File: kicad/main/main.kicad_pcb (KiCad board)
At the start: 2 copper layers, 45.7 x 35 mm, 19 parts, among them J2 Conn_01x02, J3 Conn_01x07_Pin, J4 Conn_01x04_Pin, P1 USB_C_Plug_USB2.0, SW1 MK-12C03-G015, SW3 SW_Push, SW4 SW_Push, U1 HUSB237, U2 ZX-PH2.0-WT4P

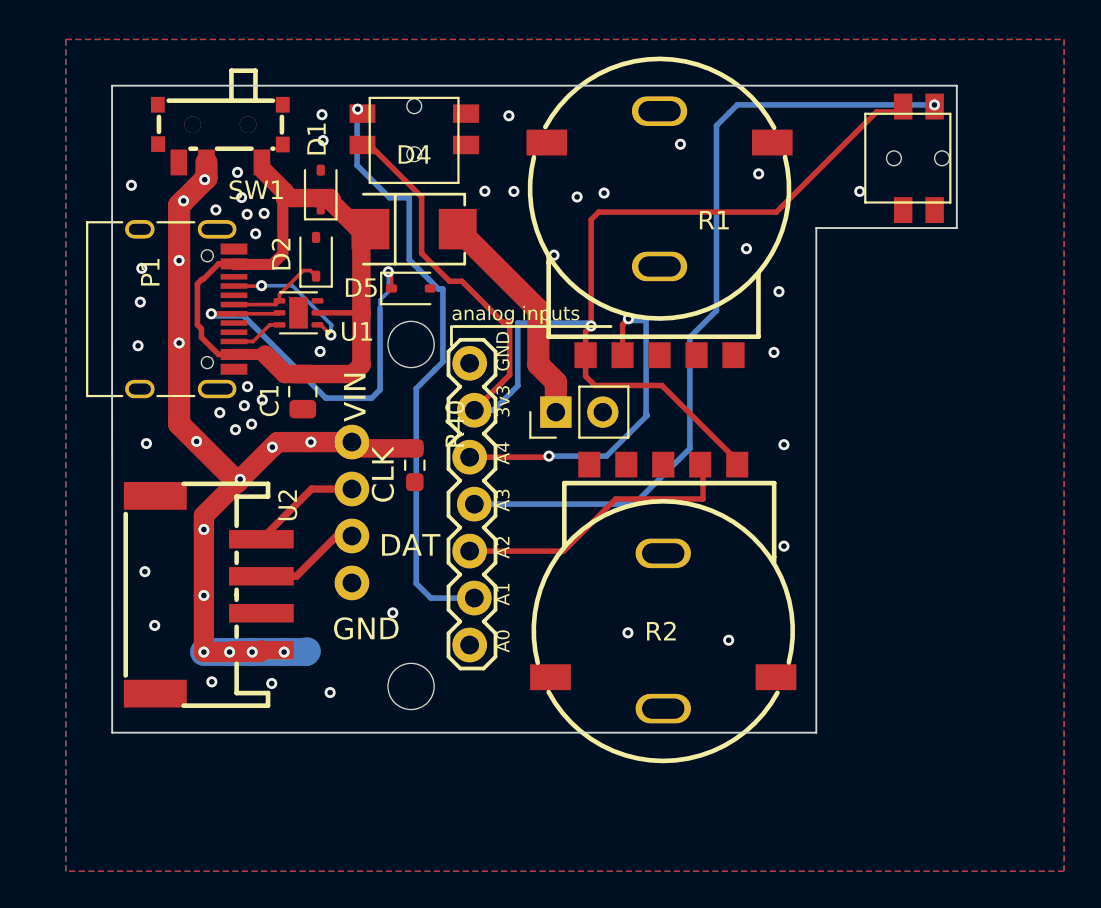
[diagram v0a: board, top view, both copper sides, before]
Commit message: Revamped PCB
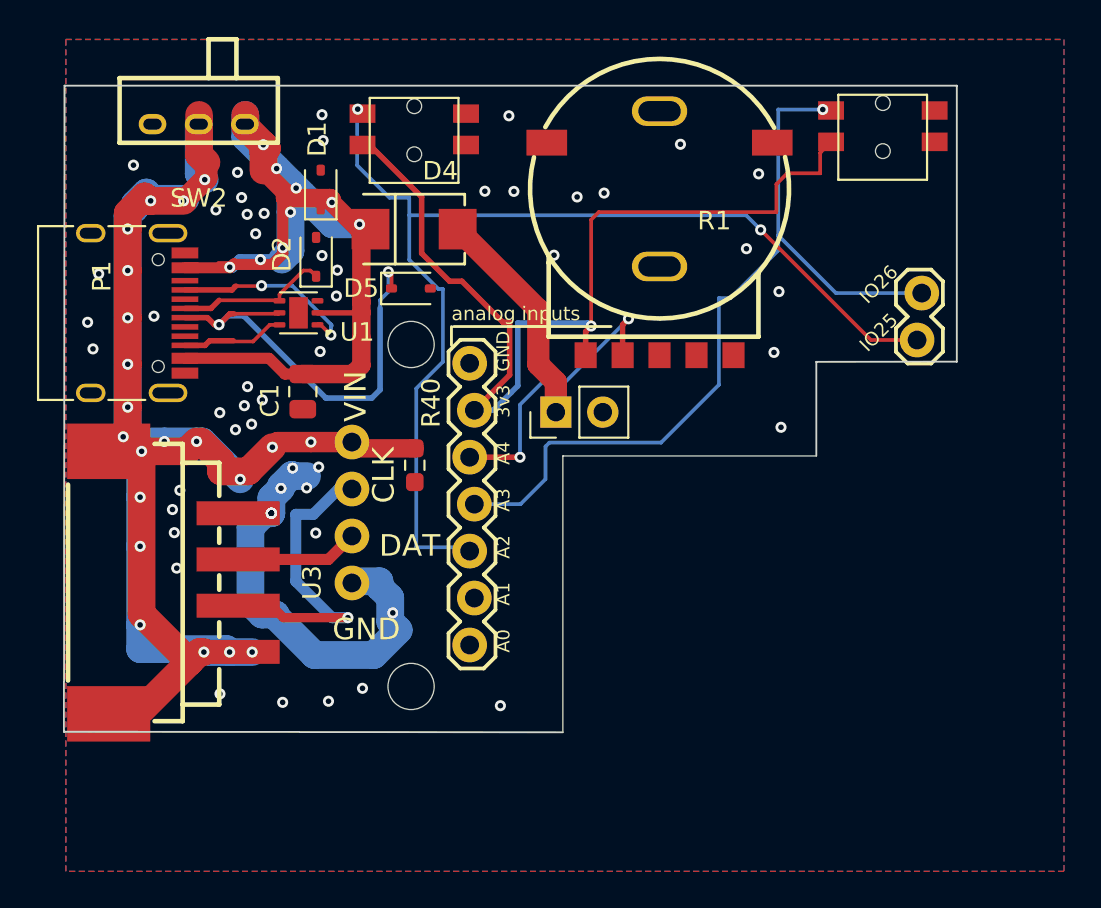
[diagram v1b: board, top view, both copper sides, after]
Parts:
- removed R2: RK10J11R0A0H, easyeda2kicad:RES-SMD_RK10J11R0A0H
- removed SW1: MK-12C03-G015, easyeda2kicad:SW-SMD_MK-12C03-G015
- removed U2: ZX-PH2.0-WT4P, easyeda2kicad:CONN-SMD_4P-P2.00_C2001RS10411M0101RC
- added J9: Conn_01x02, 1X08_LOCK_513, F.Cu at (203.7, 104.0)
- added SW2: MK-12D18-G040, easyeda2kicad:SW-TH_MK-12D18-G040, F.Cu at (164.7, 77.1)
- added U3: S4B-XH-SM4-TB-(LF)(SN), easyeda2kicad:CONN-SMD_S4B-XH-SM4-TB-LF-SN, F.Cu at (163.3, 101.9)
- moved P1 2.66 mm to (159.9, 87.3)
- moved SW4 2.54 mm to (201.7, 77.2), turned to 180 degrees
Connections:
- J3 pad 2: AIN1 -> AIN2
- J3 pad 3: AIN2 -> AIN1
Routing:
- net VIN: track 84.9 -> 115.2 mm, vias 14 -> 21
- net AIN1: track 32.4 -> 60.2 mm, vias 1 -> 2
- net GND: track 0.00 -> 23.3 mm, vias 42 -> 54
- net VBUS: track 38.3 -> 57.6 mm, vias 0 -> 9
- net AIN2: track 15.7 -> 0.00 mm
- net +3V3: track 67.9 -> 53.3 mm
- net SCK_OUT: track 6.02 -> 15.3 mm, vias 0 -> 1
- net AIN4: track 18.8 -> 15.5 mm
- net CC1: track 8.23 -> 11.1 mm
- net D+: track 5.54 -> 8.30 mm
- net CC2: track 2.83 -> 5.55 mm
- net AIN3: track 43.4 -> 45.5 mm
- net D-: track 22.5 -> 24.0 mm
- net MOSI_OUT: track 5.80 -> 4.88 mm
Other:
- board size 45.7 x 35 mm -> 48.3 x 35 mm
- board text added: "IO25"
- board text added: "IO26"
